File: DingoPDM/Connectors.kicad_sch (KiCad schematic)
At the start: 15 parts, among them J1 RedCubeTerminal, J2 USB_C_Receptacle_USB2.0, J3 1-776267-1, J4 1-776267-1, Q1 BC817-40

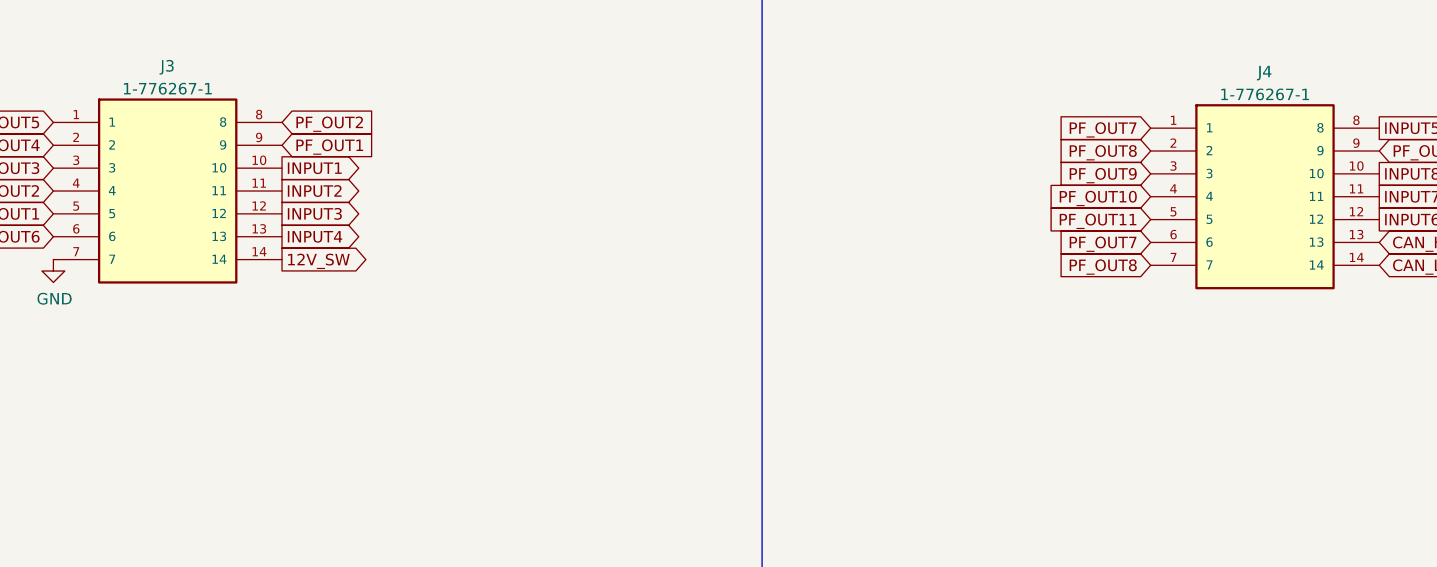
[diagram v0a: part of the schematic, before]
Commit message: layout finished
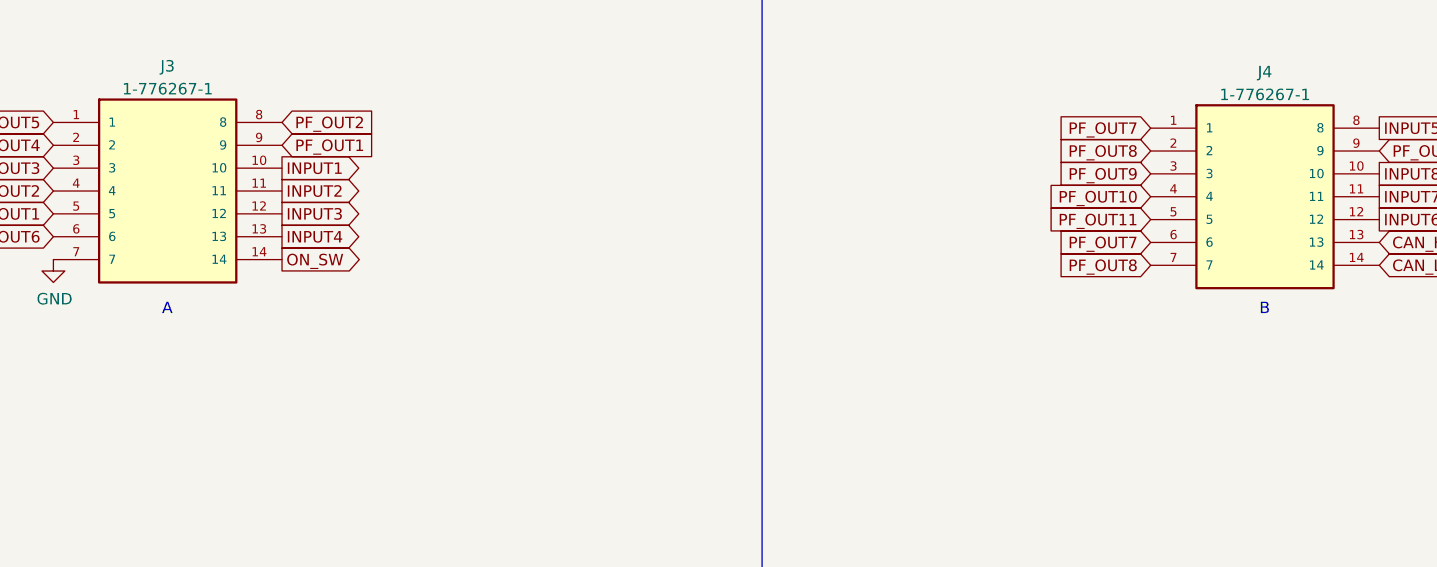
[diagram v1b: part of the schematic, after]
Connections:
- net 12V_SW renamed ON_SW
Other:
- note added: "A"
- note added: "B"
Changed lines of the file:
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@@
     (stroke (width 0) (type default) (color 0 0 0 0))
+  )
+  (text "B" (at 231.775 67.945 0)
+    (effects (font (size 1.27 1.27)) (justify left bottom))
+  )
+  (text "A" (at 109.855 67.945 0)
+    (effects (font (size 1.27 1.27)) (justify left bottom))
   )
   (text "AMPSEAL Connector" (at 178.435 100.33 0)
@@
     )
   )
-  (global_label "12V_SW" (shape output) (at 123.19 61.595 0) (fields_autoplaced)
+  (global_label "ON_SW" (shape output) (at 123.19 61.595 0) (fields_autoplaced)
     (effects (font (size 1.27 1.27)) (justify left))
-    (property "Intersheet References" "${INTERSHEET_REFS}" (id 0) (at 339.09 175.895 0)
-      (effects (font (size 1.27 1.27)) hide)
+    (property "Intersheet References" "${INTERSHEET_REFS}" (id 0) (at 131.8037 61.5156 0)
+      (effects (font (size 1.27 1.27)) (justify left) hide)
     )
   )
